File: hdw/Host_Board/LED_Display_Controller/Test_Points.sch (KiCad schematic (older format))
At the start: 10 parts

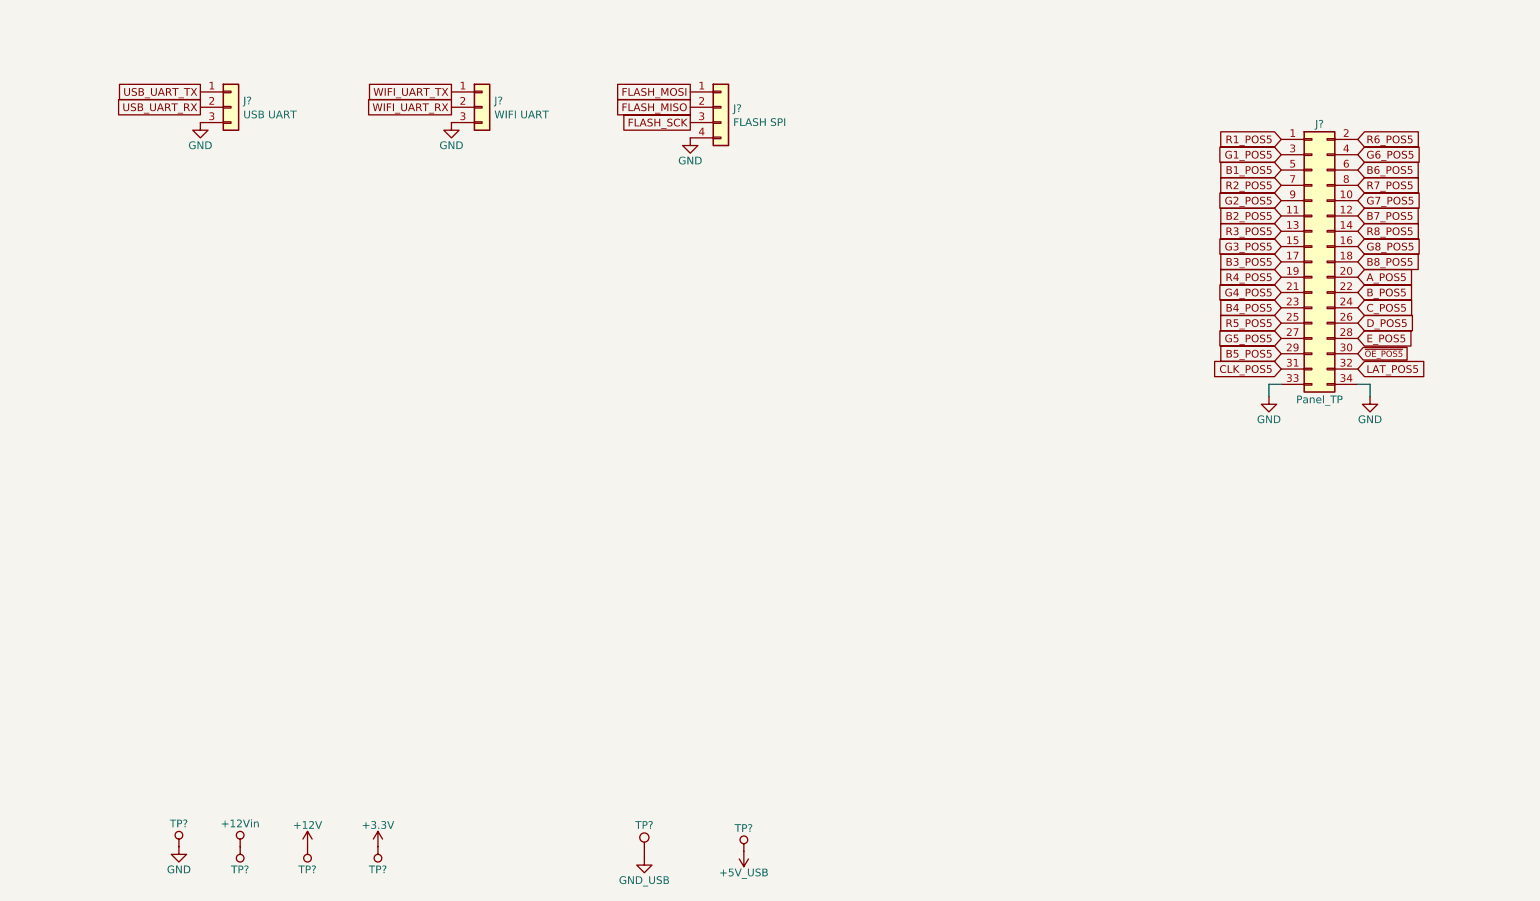
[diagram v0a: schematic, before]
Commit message: rage commit
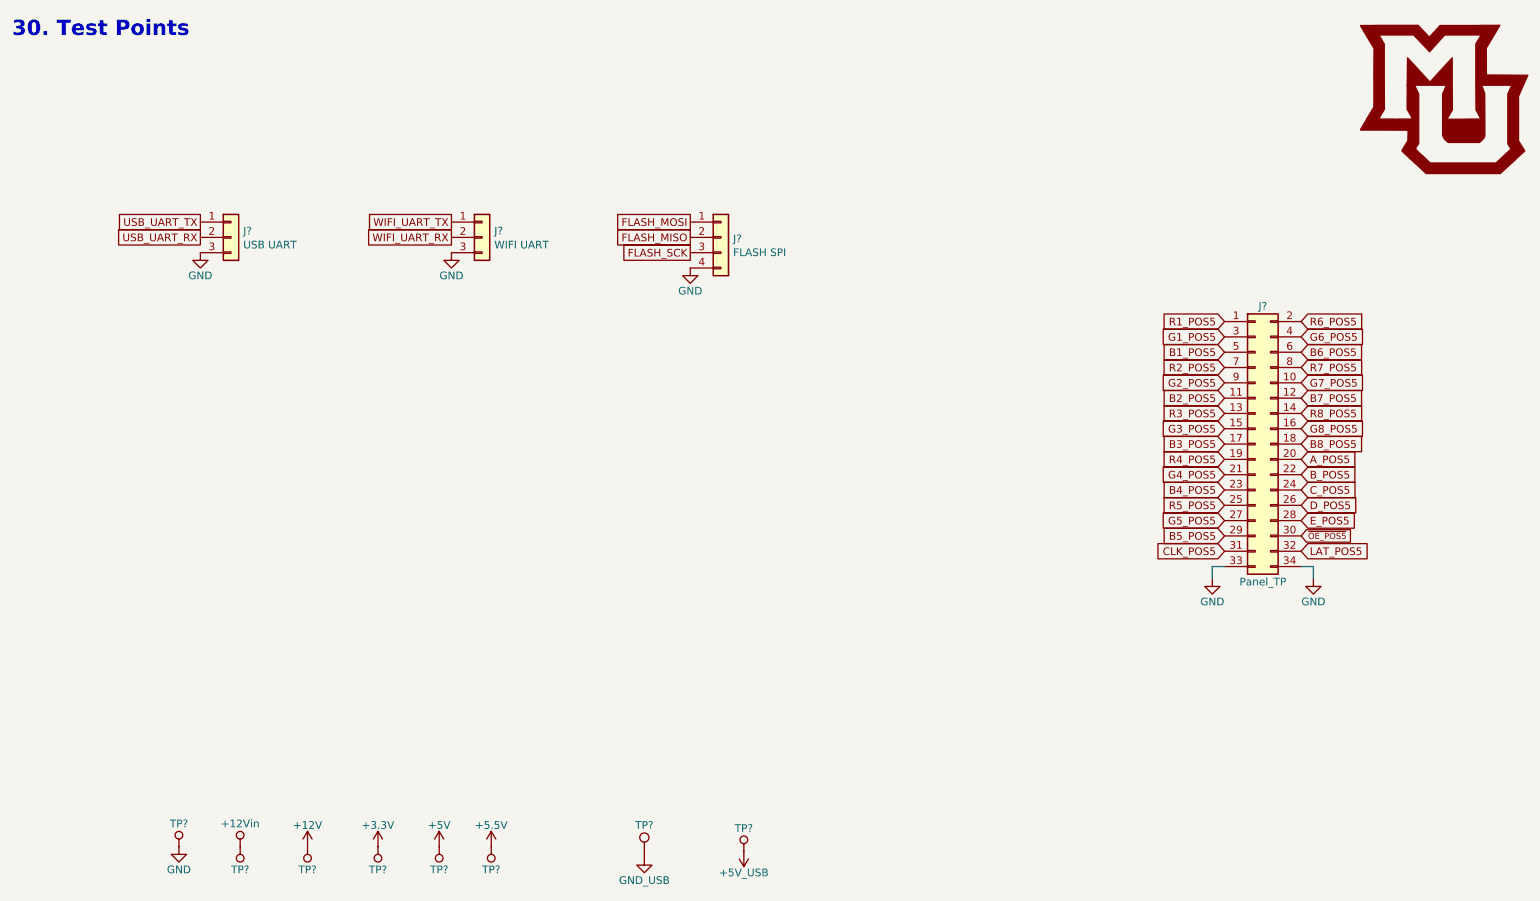
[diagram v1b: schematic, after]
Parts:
- added TP? (x2): TP, symbol Custom_Library:TP
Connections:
- new net +5.5V: TP?.1 (TP)
- new net +5V: TP?.1 (TP)
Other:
- note added: "30. Test Points"
- moved on the sheet: J?
